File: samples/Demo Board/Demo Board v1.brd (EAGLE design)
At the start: 88.9 x 50.8 mm, 56 parts

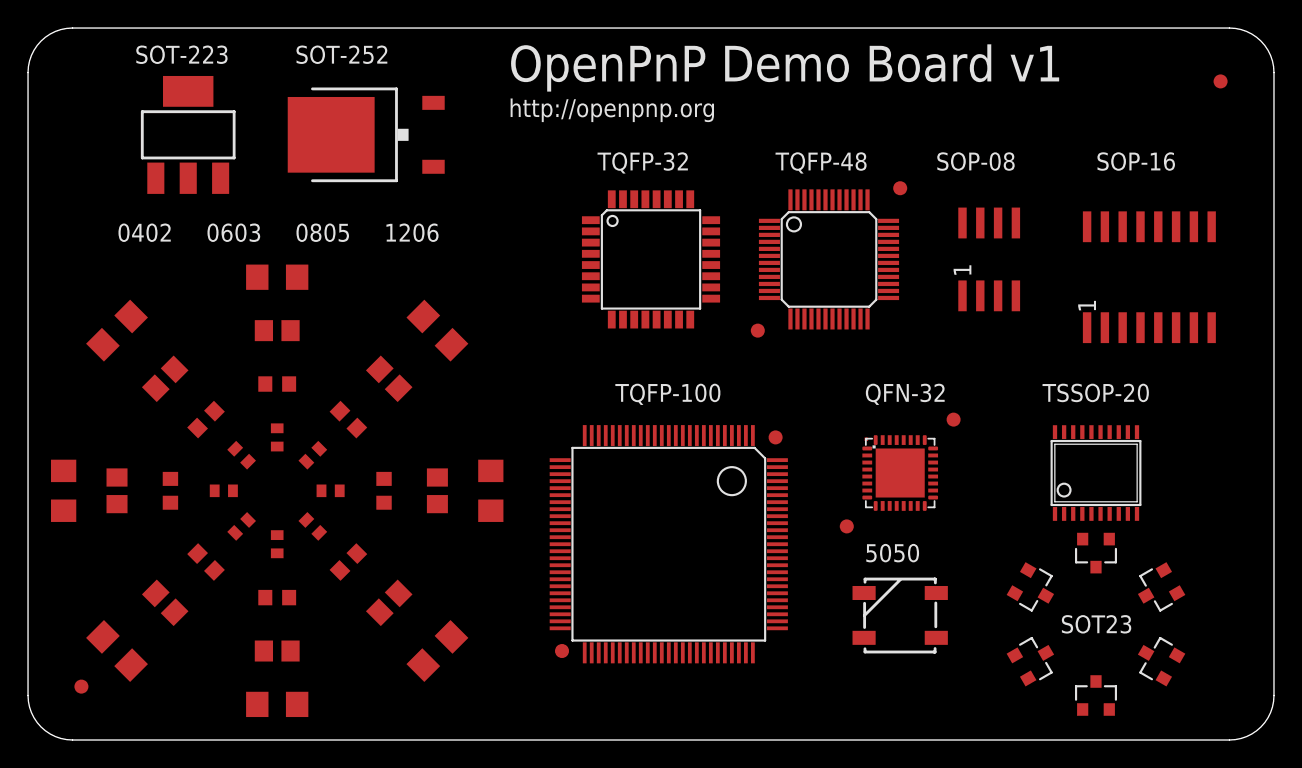
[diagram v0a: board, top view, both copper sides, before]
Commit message: Revert "Revert "Merge remote-tracking branch 'openpnp/feature/bottom-vision' into develop""
This reverts commit 273c0c9d88a1beb8fff937c1a99141638172fa66.
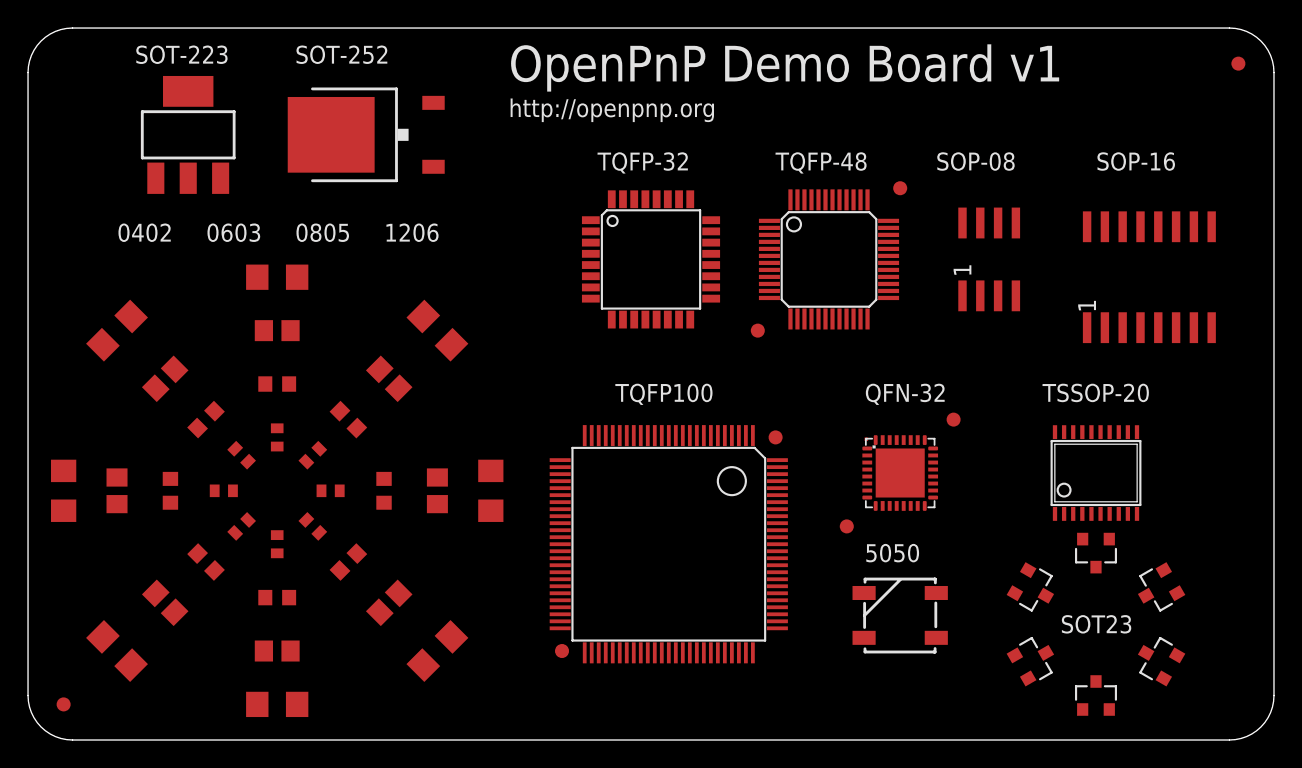
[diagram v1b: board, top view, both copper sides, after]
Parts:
- removed FID-1, FID-2: (no value), SparkFun-Aesthetics:FIDUCIAL-1X2
- added E$13, E$22: (no value), SparkFun-Aesthetics:FIDUCIAL-1X2
- renumbered 5050 to E$1, FID-3 to E$17, FID-4 to E$18, FID-5 to E$14, FID-6 to E$15, FID-7 to E$19, FID-8 to E$20, QFN-32 to E$42, R0402-1 to E$23, R0402-2 to E$27, R0402-3 to E$24, R0402-4 to E$30, R0402-5 to E$25, R0402-6 to E$28, R0402-7 to E$26, R0402-8 to E$29, R0603-1 to E$31, R0603-2 to E$37, R0603-3 to E$35, R0603-4 to E$38, R0603-5 to E$34, R0603-6 to E$39, R0603-7 to E$36, R0603-8 to E$40, R0805-1 to E$41, R0805-2 to E$55, R0805-3 to E$44, R0805-4 to E$54, R0805-5 to E$45, R0805-6 to E$48, R0805-7 to E$46, R0805-8 to E$47, R1206-1 to E$82, R1206-2 to E$7, R1206-3 to E$2, R1206-4 to E$8, R1206-5 to E$3, R1206-6 to E$9, R1206-7 to E$5, R1206-8 to E$6, SOP-08 to E$53, SOP-16 to E$4, SOT-223 to E$51, SOT-23-1 to E$60, SOT-23-2 to E$58, SOT-23-3 to E$62, SOT-23-4 to E$61, SOT-23-5 to E$56, SOT-23-6 to E$57, SOT-252 to E$52, TQFP-100 to E$16, TQFP-32 to E$11, TQFP-48 to E$12, TSSOP-20 to E$10
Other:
- board text added: "TQFP100"
- board text removed: "* FIDS are missing keepout"
- board text removed: "TQFP-100"
